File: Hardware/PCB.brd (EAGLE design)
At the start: 46.2 x 35 mm, 105 parts, among them IC1 BQ25180YBGR_BQ25180YBGR, IC2 DRV2605YZFR, IC3 BMA421, IC9 RT6160AWSC, J1 503480-2400, J2 TC2030-IDC_TC2030-IDC, J4 KH-TYPE-C-16P, Q1 20V/4.2A/52mΩ/1.4W, Q3 SI1308EDL-T1-GE3, U1 NRF52840_QF, U3 MAX17048G+T10, X1 32MHz, X2 32.768kHz

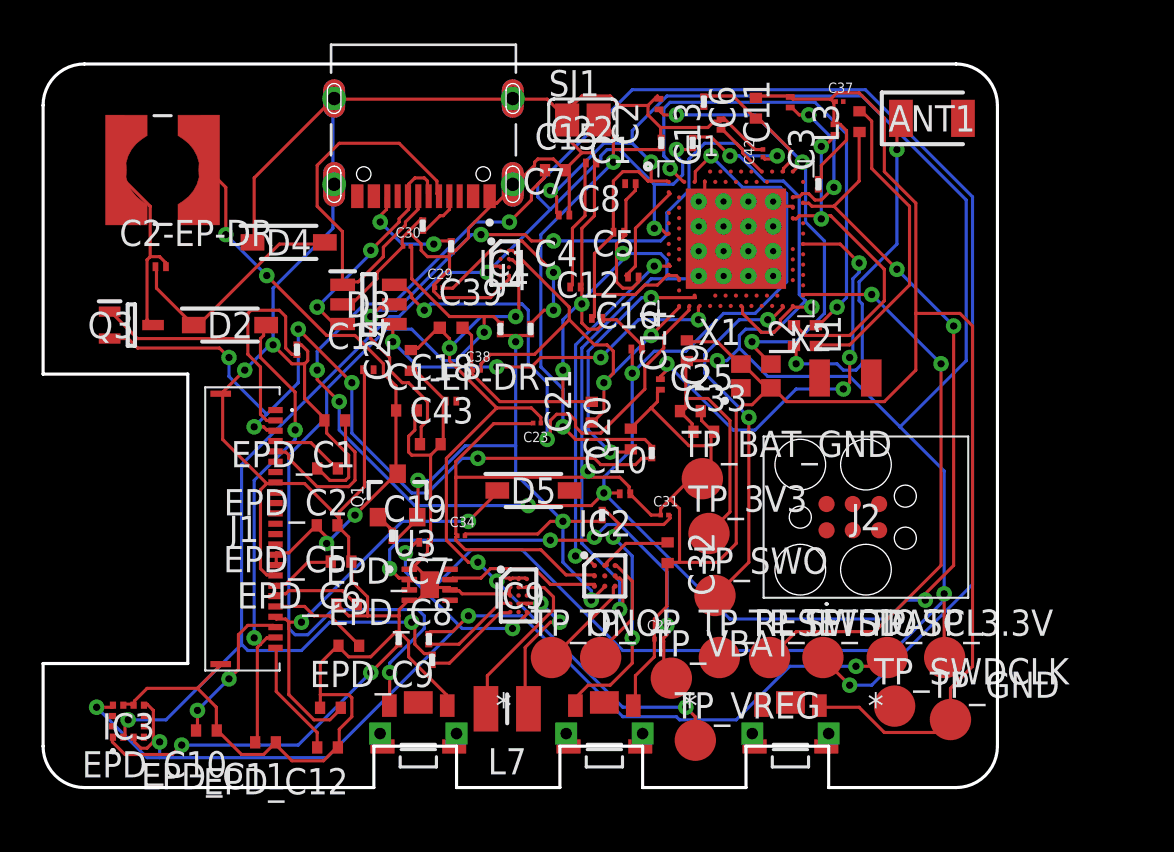
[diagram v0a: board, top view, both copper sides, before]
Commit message: second commit
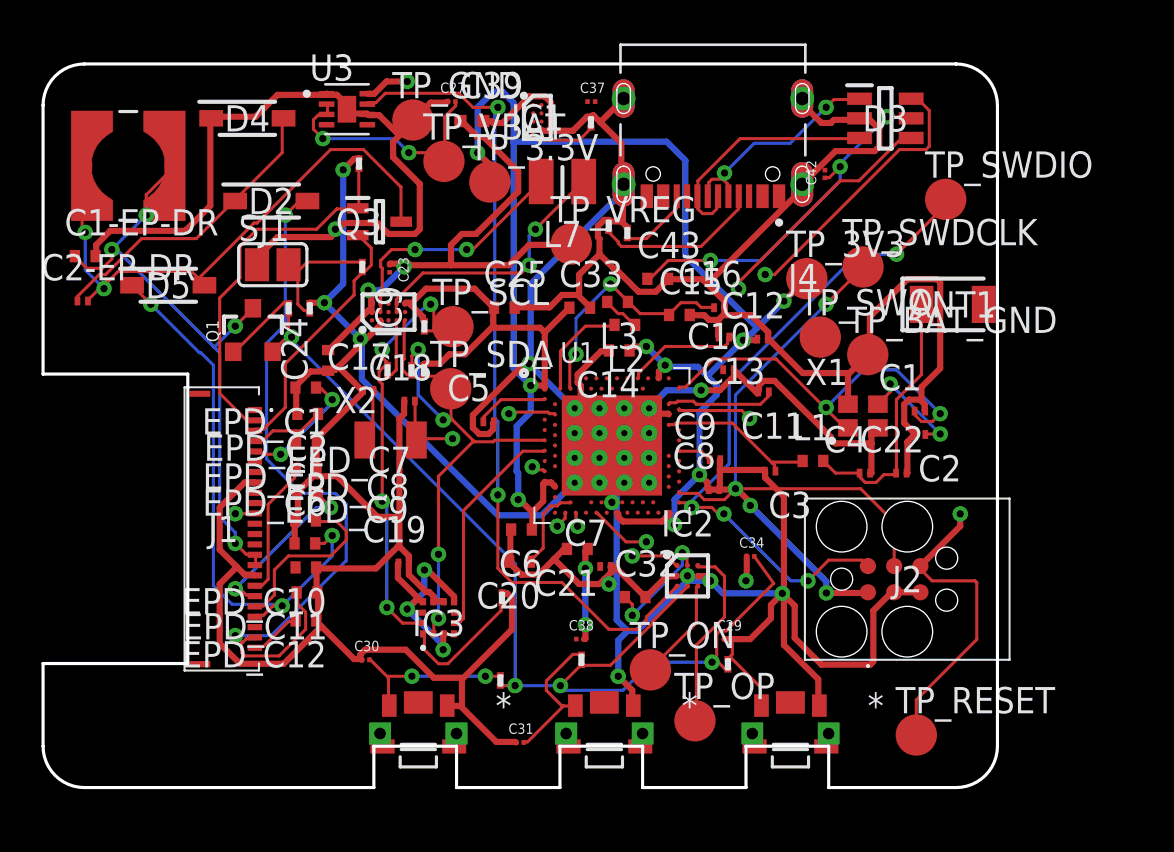
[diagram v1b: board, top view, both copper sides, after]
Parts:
- moved TP_GND 38.9 mm to (17.9, 97.3)
- moved TP_3.3V 31.8 mm to (21.6, 94.3)
- moved C27 27.9 mm to (19.8, 98.2)
- moved TP_VBAT 27.3 mm to (19.4, 95.3)
- moved D3 26.6 mm to (40.7, 97.4)
- moved TP_SCL 26.4 mm to (19.8, 87.3)
- moved L7 25.6 mm to (25.1, 94.3)
- moved TP_VREG 24.7 mm to (25.6, 91.3)
- moved TP_SWDIO 23.7 mm to (43.7, 93.4)
- moved U3 23.3 mm to (14.7, 97.8)
- moved C6 23.3 mm to (23.1, 77.5), turned to 180 degrees
- moved X2 22.2 mm to (16.8, 81.8)
- moved TP_SDA 22.2 mm to (19.7, 84.3)
- moved C29 22.0 mm to (33.1, 72.2)
- moved TP_SWDCLK 21.3 mm to (39.7, 90.2)
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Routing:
- net SDA/2.4C: track 117.4 -> 23.3 mm, vias 6 -> 4
- net DEC4_6: track 108.0 -> 24.9 mm, vias 10 -> 3
- net 3V3/2.4A: track 184.8 -> 119.8 mm, vias 10 -> 14
- net RESET: track 0.00 -> 34.8 mm, vias 0 -> 2
- net P0.13/1.5D: track 42.2 -> 8.18 mm
- net SCL/1.4C: track 7.60 -> 40.1 mm, vias 0 -> 2
- net SDA/1.4C: track 0.00 -> 31.7 mm, vias 0 -> 2
- net GND: track 399.6 -> 370.7 mm, vias 7 -> 12
- net SWDCLK: track 0.00 -> 26.9 mm, vias 0 -> 2
- net RESE: track 39.1 -> 12.3 mm, vias 5 -> 0
- net EPD_DC: track 0.00 -> 26.0 mm, vias 0 -> 2
- net N$10: track 21.1 -> 1.67 mm, vias 4 -> 0
- net N$13: track 0.00 -> 19.1 mm, vias 0 -> 2
- net N$15: track 9.46 -> 28.3 mm, vias 0 -> 2
- net N$17: track 23.5 -> 4.96 mm, vias 2 -> 0
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- added copper zone on layer 2, net GND
